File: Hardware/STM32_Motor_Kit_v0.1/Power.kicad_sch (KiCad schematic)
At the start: 66 parts, among them J1 Conn_01x02_Male, U2 AMS111733TR-HT, U3 LMV358IDRG4, U4 TPS54331DR, U5 MC78M15CDTRKG-

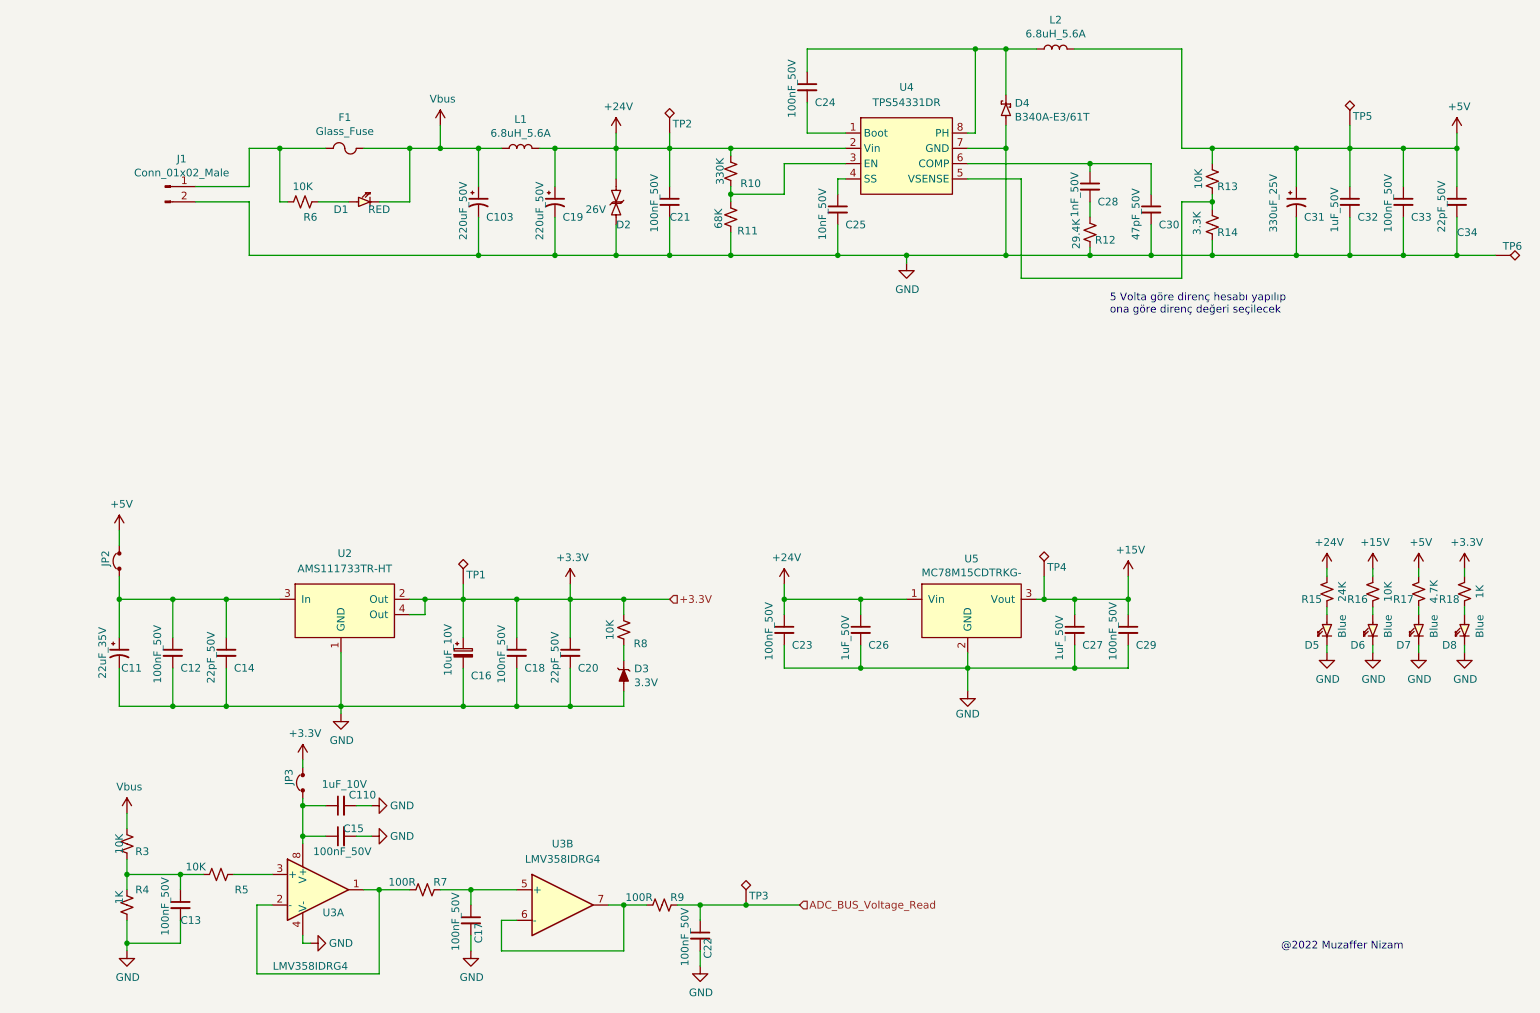
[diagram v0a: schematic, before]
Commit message: 16.09.2024
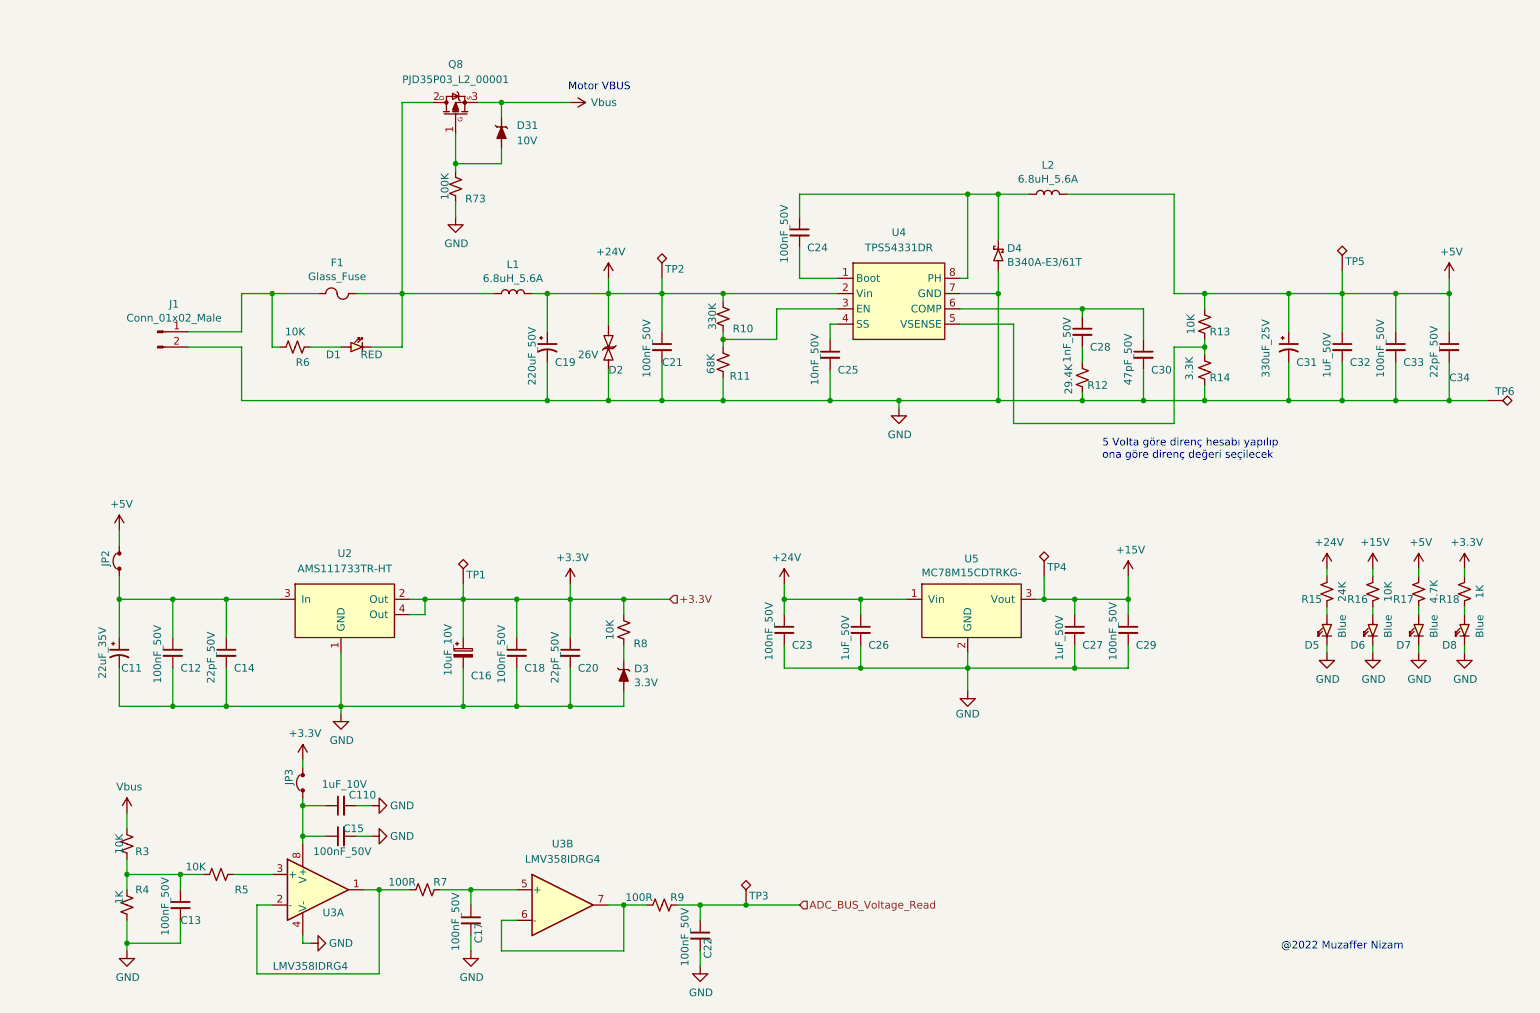
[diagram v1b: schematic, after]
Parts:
- removed C103: 220uF_50V, AKE_Capacitor_TH:CP_Radial_D10.0mm_P5.00mm, symbol AKE_Capacitor:Capacitor_Polarised
- added D31: 10V, AKE_Diode_SMD:SMA, symbol AKE_Diode:Diode_Zener
- added Q8: PJD35P03_L2_00001, AKE_Mosfet_SMD:DPAK_123, symbol AKE_MOSFET:PJD35P03_L2_00001
- added R73: 100K, AKE_Resistor_SMD:RES_1206, symbol AKE_Resistor:Resistor_US
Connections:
- net GND: now also R73.1
- net Vbus: now also D31.1, Q8.3 (S); no longer D1.1, F1.2, L1.1
- new net: D31.2, Q8.1 (G), R73.2
- new net: D1.1, F1.2, L1.1, Q8.2 (D)
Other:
- note added: "Motor VBUS"
- moved on the sheet: C19, C21, C24, C25, C28, C30, C31, C32, C33, C34, D1, D2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

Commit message: 12.01.2025
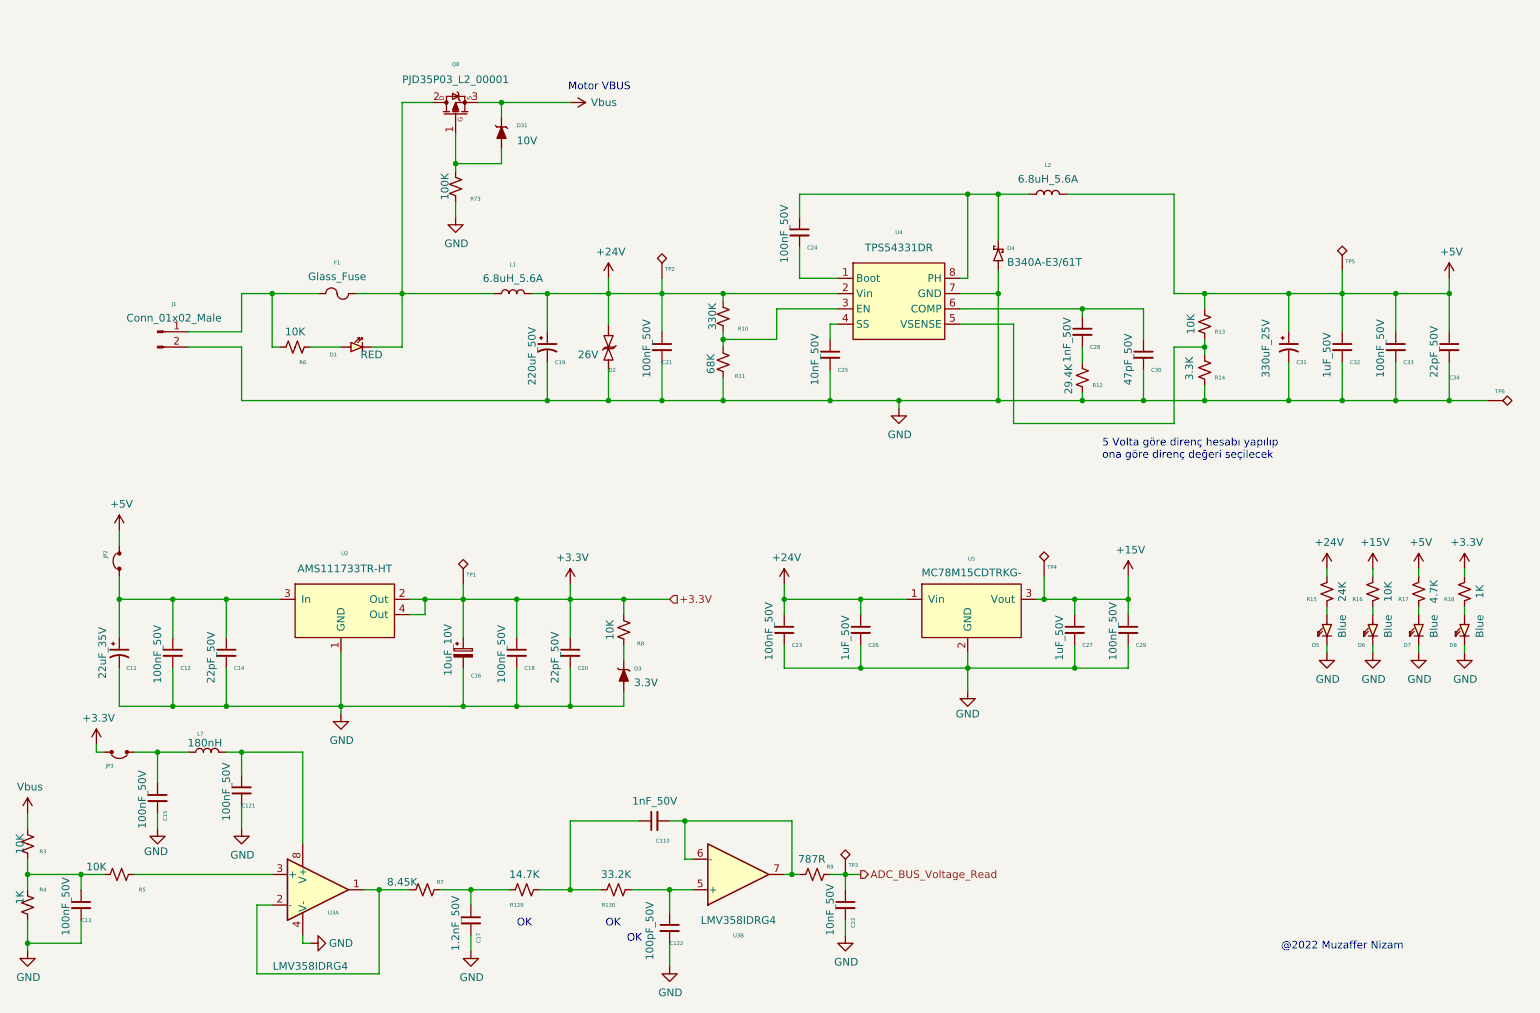
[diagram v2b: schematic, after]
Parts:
- added C121: 100nF_50V, AKE_Capacitor_SMD:CAP_0603, symbol AKE_Capacitor:Capacitor_UnPolarised
- added C122: 100pF_50V, AKE_Capacitor_SMD:CAP_0603, symbol AKE_Capacitor:Capacitor_UnPolarised
- added L7: 180nH, AKE_Inductor_SMD:IND_0603, symbol AKE_Inductor:Inductor
- added R129: 14.7K, AKE_Resistor_SMD:RES_0603, symbol AKE_Resistor:Resistor_US
- added R130: 33.2K, AKE_Resistor_SMD:RES_0603, symbol AKE_Resistor:Resistor_US
- C110: value 1uF_10V -> 1nF_50V
- C17: value 100nF_50V -> 1.2nF_50V
- C22: value 100nF_50V -> 10nF_50V
- R7: value 100R -> 8.45K
- R9: value 100R -> 787R
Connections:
- net GND: now also C121.2, C122.2; no longer C110.2
- net at R9.2, U3.6 (-), U3.7: now also C110.2
- net at C15.1, JP3.1 (A): now also L7.1; no longer C110.1, U3.8 (V+)
- net at C17.1, R7.1: now also R129.2; no longer U3.5 (+)
- new net: C121.1, L7.2, U3.8 (V+)
- new net: C110.1, R129.1, R130.2
- new net: C122.1, R130.1, U3.5 (+)
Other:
- note added: "OK"
- moved on the sheet: C13, C15, C22, JP3, R3, R4, R5, R9, TP3, U3B
